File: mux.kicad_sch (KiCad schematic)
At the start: 22 parts, among them M1 SN74LV4051ADYYR, M10 SN74LV4051ADYYR, M11 SN74LV4051ADYYR, M2 SN74LV4051ADYYR, M3 SN74LV4051ADYYR, M4 SN74LV4051ADYYR, M5 SN74LV4051ADYYR, M6 SN74LV4051ADYYR, M7 SN74LV4051ADYYR, M8 SN74LV4051ADYYR, M9 SN74LV4051ADYYR

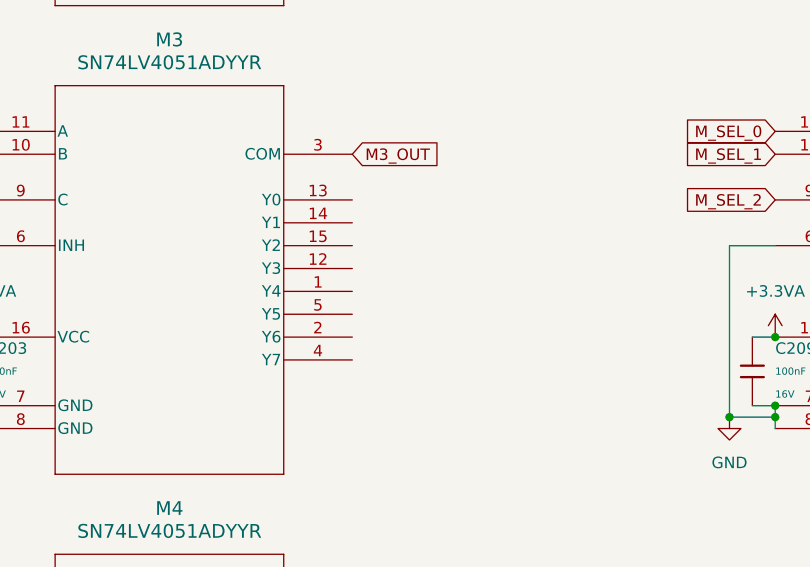
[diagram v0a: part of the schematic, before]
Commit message: continue sensor out
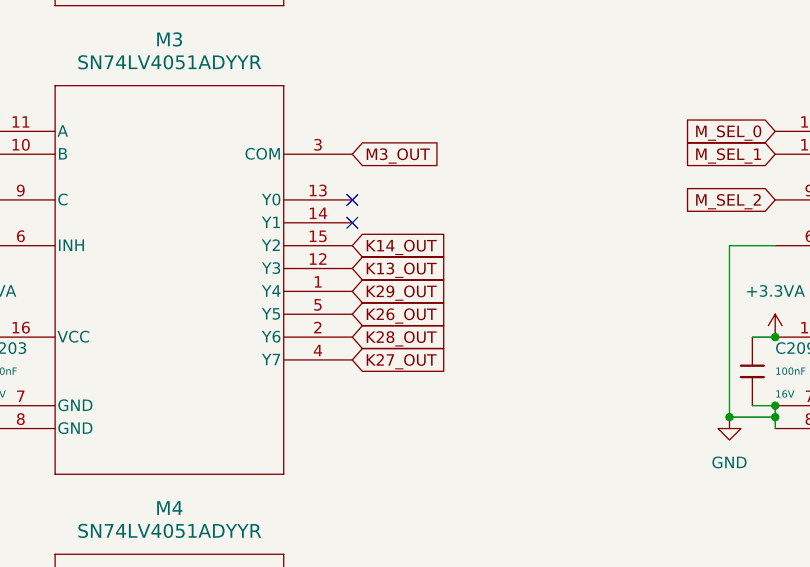
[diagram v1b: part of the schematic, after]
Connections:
- net K26_OUT: now also M3.5 (Y5)
- net K29_OUT: now reaches M3.1 (Y4)
- net K13_OUT: now reaches M3.12 (Y3)
- net K14_OUT: now reaches M3.15 (Y2)
- net K28_OUT: now reaches M3.2 (Y6)
- net K27_OUT: now reaches M3.4 (Y7)
- no-connect marks 4 -> 6
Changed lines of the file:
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@@
 		(at 69.85 195.58)
 	)
+	(no_connect
+		(at 69.85 140.97)
+	)
+	(no_connect
+		(at 69.85 143.51)
+	)
 	(wire
 		(pts
@@
 		)
 	)
+	(global_label "K13_OUT"
+		(shape input)
+		(at 69.85 148.59 0)
+		(fields_autoplaced yes)
+		(effects
+			(font
+				(size 1.27 1.27)
+			)
+			(justify left)
+		)
+		(property "Intersheetrefs" "${INTERSHEET_REFS}"
+			(at 81.1204 148.59 0)
+			(effects
+				(font
+					(size 1.27 1.27)
+				)
+				(justify left)
+				(hide yes)
+			)
+		)
+	)
 	(global_label "K34_OUT"
 		(shape input)
@@
 		)
 	)
+	(global_label "K27_OUT"
+		(shape input)
+		(at 69.85 158.75 0)
+		(fields_autoplaced yes)
+		(effects
+			(font
+				(size 1.27 1.27)
+			)
+			(justify left)
+		)
+		(property "Intersheetrefs" "${INTERSHEET_REFS}"
+			(at 81.1204 158.75 0)
+			(effects
+				(font
+					(size 1.27 1.27)
+				)
+				(justify left)
+				(hide yes)
+			)
+		)
+	)
 	(global_label "M_SEL_1"
 		(shape input)
@@
 		)
 	)
+	(global_label "K28_OUT"
+		(shape input)
+		(at 69.85 156.21 0)
+		(fields_autoplaced yes)
+		(effects
+			(font
+				(size 1.27 1.27)
+			)
+			(justify left)
+		)
+		(property "Intersheetrefs" "${INTERSHEET_REFS}"
+			(at 81.1204 156.21 0)
+			(effects
+				(font
+					(size 1.27 1.27)
+				)
+				(justify left)
+				(hide yes)
+			)
+		)
+	)
 	(global_label "M_SEL_1"
 		(shape input)
@@
 		)
 	)
+	(global_label "K14_OUT"
+		(shape input)
+		(at 69.85 146.05 0)
+		(fields_autoplaced yes)
+		(effects
+			(font
+				(size 1.27 1.27)
+			)
+			(justify left)
+		)
+		(property "Intersheetrefs" "${INTERSHEET_REFS}"
+			(at 81.1204 146.05 0)
+			(effects
+				(font
+					(size 1.27 1.27)
+				)
+				(justify left)
+				(hide yes)
+			)
+		)
+	)
 	(global_label "K45_OUT"
 		(shape input)
@@
 		)
 	)
+	(global_label "K26_OUT"
+		(shape input)
+		(at 69.85 153.67 0)
+		(fields_autoplaced yes)
+		(effects
+			(font
+				(size 1.27 1.27)
+			)
+			(justify left)
+		)
+		(property "Intersheetrefs" "${INTERSHEET_REFS}"
+			(at 81.1204 153.67 0)
+			(effects
+				(font
+					(size 1.27 1.27)
+				)
+				(justify left)
+				(hide yes)
+			)
+		)
+	)
 	(global_label "M3_OUT"
 		(shape input)
@@
 			(effects
 				(font
+					(size 1.27 1.27)
+				)
+				(justify left)
+				(hide yes)
+			)
+		)
+	)
+	(global_label "K29_OUT"
+		(shape input)
+		(at 69.85 151.13 0)
+		(fields_autoplaced yes)
+		(effects
+			(font
+				(size 1.27 1.27)
+			)
+			(justify left)
+		)
+		(property "Intersheetrefs" "${INTERSHEET_REFS}"
+			(at 81.1204 151.13 0)
+			(effects
+				(font
